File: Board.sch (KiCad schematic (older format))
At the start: 5 parts, among them P1 Relay 1, P2 Relay 2, P3 Relay 3, P4 Relay 4

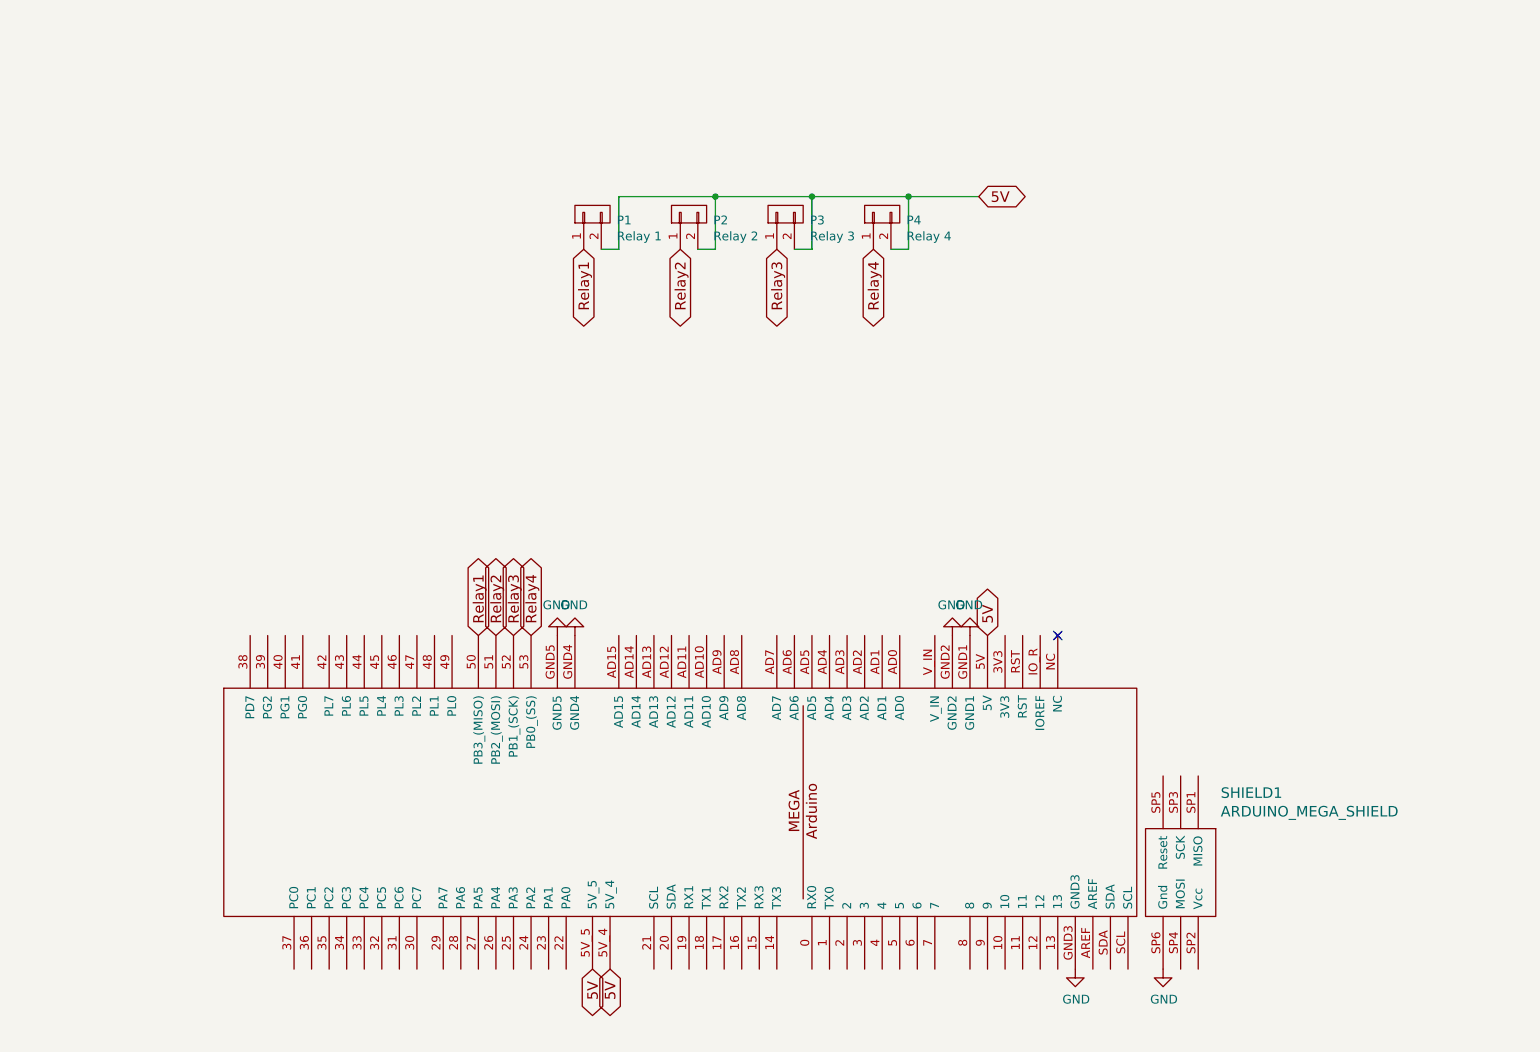
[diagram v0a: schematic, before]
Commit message: Pins are in
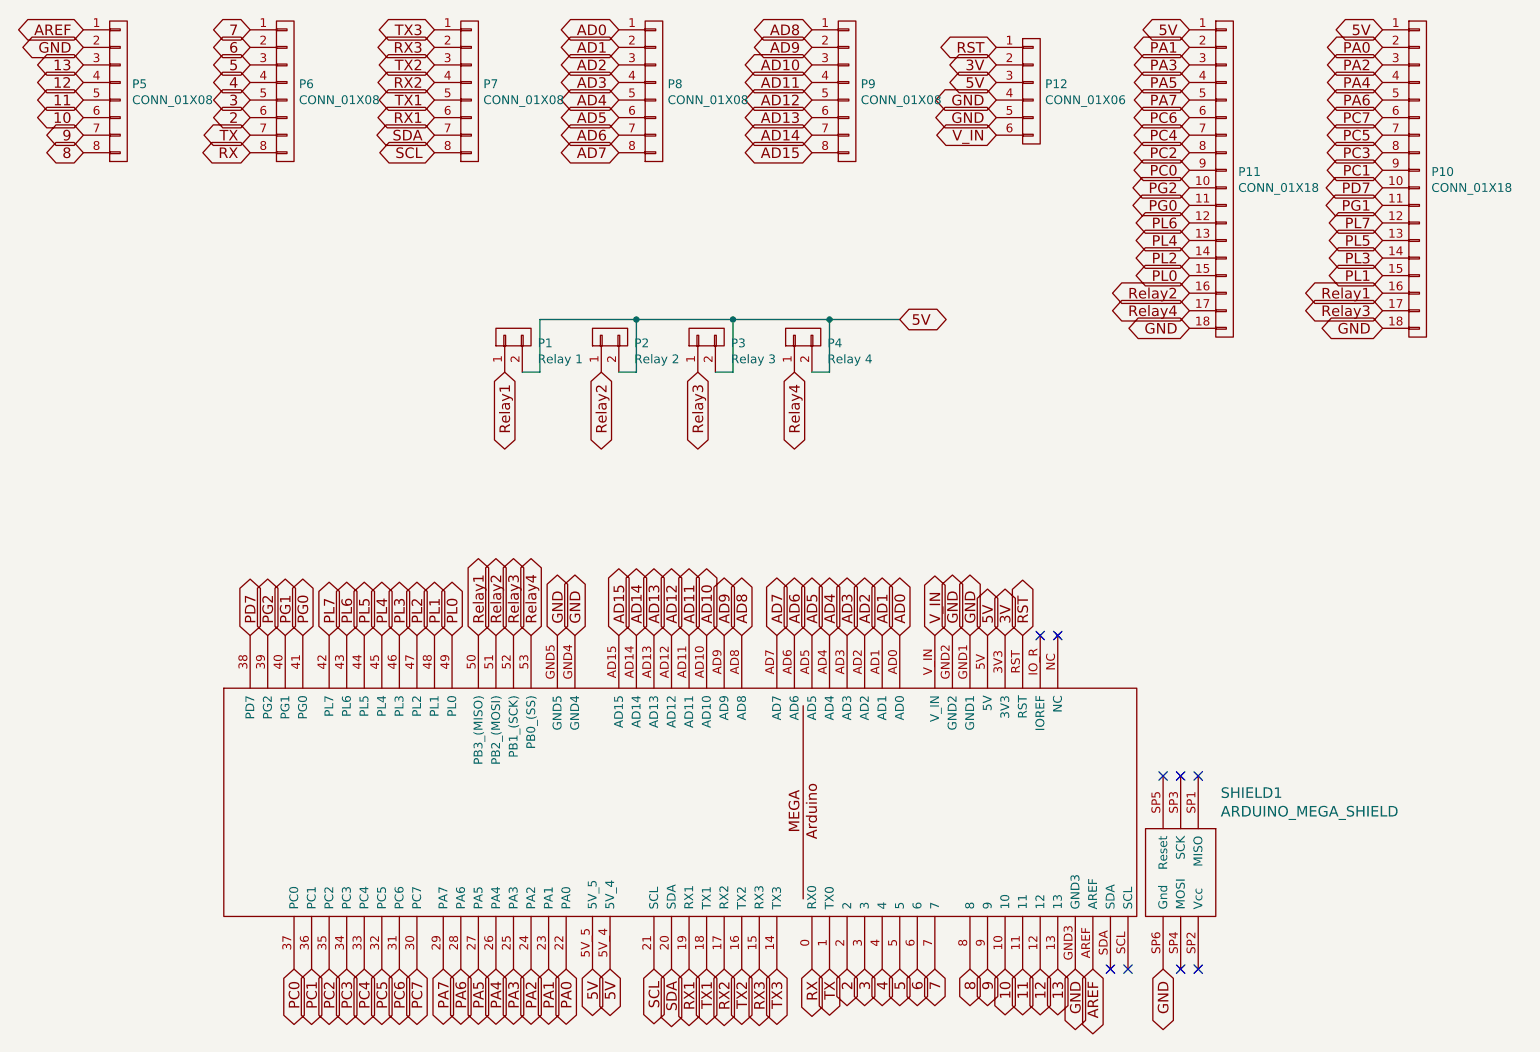
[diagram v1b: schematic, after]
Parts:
- added P10, P11: CONN_01X18, Pin_Headers:Pin_Header_Straight_1x18, symbol CONN_01X18
- added P12: CONN_01X06, Pin_Headers:Pin_Header_Straight_1x06, symbol CONN_01X06
- added P5, P6, P7, P8, P9: CONN_01X08, Pin_Headers:Pin_Header_Straight_1x08, symbol CONN_01X08
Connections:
- net 5V: now also P10.1 (P1), P11.1 (P1), P12.3 (P3)
- net GND: now also P10.18 (P18), P11.18 (P18), P12.4 (P4), P12.5 (P5), P5.2 (P2)
- net Relay1: now also P10.16 (P16)
- net Relay2: now also P11.16 (P16)
- net Relay3: now also P10.17 (P17)
- net Relay4: now also P11.17 (P17)
- net RX: now reaches SHIELD1.0 (RX0)
- net RX: now also P6.8 (P8)
- net TX: now reaches SHIELD1.1 (TX0)
- net TX: now also P6.7 (P7)
- net 10: now reaches SHIELD1.10
- net 10: now also P5.6 (P6)
- net 11: now reaches SHIELD1.11
- net 11: now also P5.5 (P5)
- net 12: now reaches SHIELD1.12
- net 12: now also P5.4 (P4)
- net 13: now reaches SHIELD1.13
- net 13: now also P5.3 (P3)
- net TX3: now reaches SHIELD1.14 (TX3)
- net TX3: now also P7.1 (P1)
- net RX3: now reaches SHIELD1.15 (RX3)
- net RX3: now also P7.2 (P2)
- net TX2: now reaches SHIELD1.16 (TX2)
- net TX2: now also P7.3 (P3)
- net RX2: now reaches SHIELD1.17 (RX2)
- net RX2: now also P7.4 (P4)
- net TX1: now reaches SHIELD1.18 (TX1)
- net TX1: now also P7.5 (P5)
- net RX1: now reaches SHIELD1.19 (RX1)
- net RX1: now also P7.6 (P6)
- net 2: now reaches SHIELD1.2
- net 2: now also P6.6 (P6)
- net SDA: now reaches SHIELD1.20 (SDA)
- net SDA: now also P7.7 (P7)
- net SCL: now reaches SHIELD1.21 (SCL)
- net SCL: now also P7.8 (P8)
- net PA0: now reaches SHIELD1.22 (PA0)
- net PA0: now also P10.2 (P2)
- net PA1: now reaches SHIELD1.23 (PA1)
- net PA1: now also P11.2 (P2)
- net PA2: now reaches SHIELD1.24 (PA2)
- net PA2: now also P10.3 (P3)
- net PA3: now reaches SHIELD1.25 (PA3)
- net PA3: now also P11.3 (P3)
- net PA4: now reaches SHIELD1.26 (PA4)
- net PA4: now also P10.4 (P4)
- net PA5: now reaches SHIELD1.27 (PA5)
- net PA5: now also P11.4 (P4)
- net PA6: now reaches SHIELD1.28 (PA6)
- net PA6: now also P10.5 (P5)
- net PA7: now reaches SHIELD1.29 (PA7)
- net PA7: now also P11.5 (P5)
- net 3: now reaches SHIELD1.3
- net 3: now also P6.5 (P5)
- net PC7: now reaches SHIELD1.30 (PC7)
- net PC7: now also P10.6 (P6)
- net PC6: now reaches SHIELD1.31 (PC6)
- net PC6: now also P11.6 (P6)
- net PC5: now reaches SHIELD1.32 (PC5)
- net PC5: now also P10.7 (P7)
- net PC4: now reaches SHIELD1.33 (PC4)
- net PC4: now also P11.7 (P7)
- net PC3: now reaches SHIELD1.34 (PC3)
- net PC3: now also P10.8 (P8)
- net PC2: now reaches SHIELD1.35 (PC2)
- net PC2: now also P11.8 (P8)
- net PC1: now reaches SHIELD1.36 (PC1)
- net PC1: now also P10.9 (P9)
- net PC0: now reaches SHIELD1.37 (PC0)
- net PC0: now also P11.9 (P9)
- net PD7: now reaches SHIELD1.38 (PD7)
- net PD7: now also P10.10 (P10)
- net PG2: now reaches SHIELD1.39 (PG2)
- net PG2: now also P11.10 (P10)
- net 3V: now reaches SHIELD1.3V3
- net 3V: now also P12.2 (P2)
- net 4: now reaches SHIELD1.4
- net 4: now also P6.4 (P4)
- net PG1: now reaches SHIELD1.40 (PG1)
- net PG1: now also P10.11 (P11)
- net PG0: now reaches SHIELD1.41 (PG0)
- net PG0: now also P11.11 (P11)
- net PL7: now reaches SHIELD1.42 (PL7)
- net PL7: now also P10.12 (P12)
- net PL6: now reaches SHIELD1.43 (PL6)
- net PL6: now also P11.12 (P12)
- net PL5: now reaches SHIELD1.44 (PL5)
- net PL5: now also P10.13 (P13)
- net PL4: now reaches SHIELD1.45 (PL4)
- net PL4: now also P11.13 (P13)
- net PL3: now reaches SHIELD1.46 (PL3)
- net PL3: now also P10.14 (P14)
- net PL2: now reaches SHIELD1.47 (PL2)
- net PL2: now also P11.14 (P14)
- net PL1: now reaches SHIELD1.48 (PL1)
- net PL1: now also P10.15 (P15)
- net PL0: now reaches SHIELD1.49 (PL0)
- net PL0: now also P11.15 (P15)
- net 5: now reaches SHIELD1.5
- net 5: now also P6.3 (P3)
- net 6: now reaches SHIELD1.6
- net 6: now also P6.2 (P2)
- net 7: now reaches SHIELD1.7
- net 7: now also P6.1 (P1)
- net 8: now reaches SHIELD1.8
- net 8: now also P5.8 (P8)
- net 9: now reaches SHIELD1.9
- net 9: now also P5.7 (P7)
- net AD0: now reaches SHIELD1.AD0
- net AD0: now also P8.1 (P1)
- net AD1: now reaches SHIELD1.AD1
- net AD1: now also P8.2 (P2)
- net AD10: now reaches SHIELD1.AD10
- net AD10: now also P9.3 (P3)
- net AD11: now reaches SHIELD1.AD11
- net AD11: now also P9.4 (P4)
- net AD12: now reaches SHIELD1.AD12
- net AD12: now also P9.5 (P5)
- net AD13: now reaches SHIELD1.AD13
- net AD13: now also P9.6 (P6)
- net AD14: now reaches SHIELD1.AD14
- net AD14: now also P9.7 (P7)
- net AD15: now reaches SHIELD1.AD15
- net AD15: now also P9.8 (P8)
- net AD2: now reaches SHIELD1.AD2
- net AD2: now also P8.3 (P3)
- net AD3: now reaches SHIELD1.AD3
- net AD3: now also P8.4 (P4)
- net AD4: now reaches SHIELD1.AD4
- net AD4: now also P8.5 (P5)
- net AD5: now reaches SHIELD1.AD5
- net AD5: now also P8.6 (P6)
- net AD6: now reaches SHIELD1.AD6
- net AD6: now also P8.7 (P7)
- net AD7: now reaches SHIELD1.AD7
- net AD7: now also P8.8 (P8)
- net AD8: now reaches SHIELD1.AD8
- net AD8: now also P9.1 (P1)
- net AD9: now reaches SHIELD1.AD9
- net AD9: now also P9.2 (P2)
- net AREF: now reaches SHIELD1.AREF
- net AREF: now also P5.1 (P1)
- net RST: now reaches SHIELD1.RST
- net RST: now also P12.1 (P1)
- net V_IN: now reaches SHIELD1.V_IN
- net V_IN: now also P12.6 (P6)
- no-connect marks 1 -> 9
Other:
- moved on the sheet: P1, P2, P3, P4
